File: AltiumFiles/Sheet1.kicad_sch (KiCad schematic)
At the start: 57 parts, among them J1 PJ-002A, U1 LM7805CT, U1A SS-104-G-2, U1RT SS-104-G-2, U2RT SS-104-G-2, Y1 ECS-100-18-1

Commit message: Kod za main
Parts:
- removed SW?: 2-1825910-7, FP-2-1825910-7-MFG, symbol Sheet1-altium-import:root_0_b8895f3f4cefb76e1819d2863dba89b
- added SW?: 2-1825910-7, FP-2-1825910-7-MFG, symbol Sheet1-altium-import:root_0_b8895f3f4cefb76e1819d2863dba89b
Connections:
- net GND: now also SW?.1, SW?.2, SW?.3, SW?.4

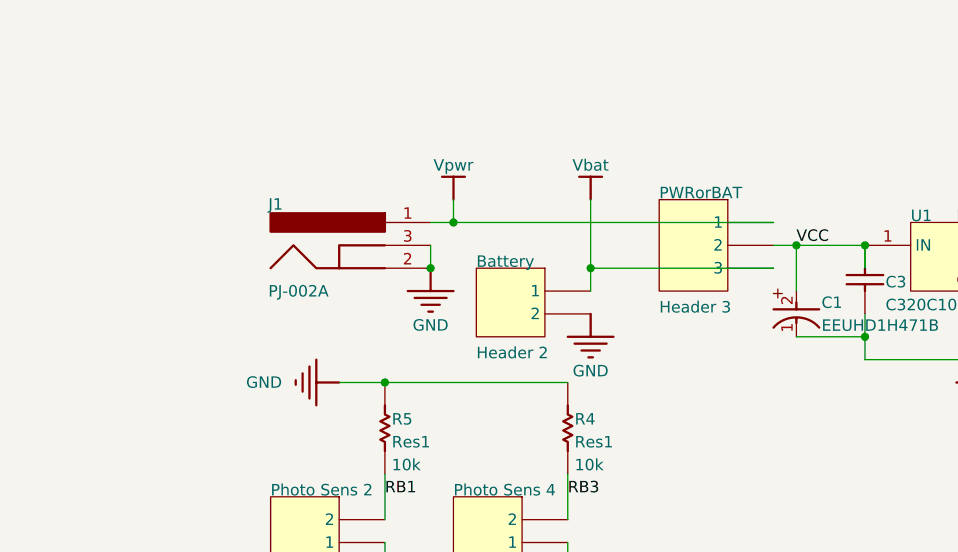
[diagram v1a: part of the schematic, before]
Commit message: End
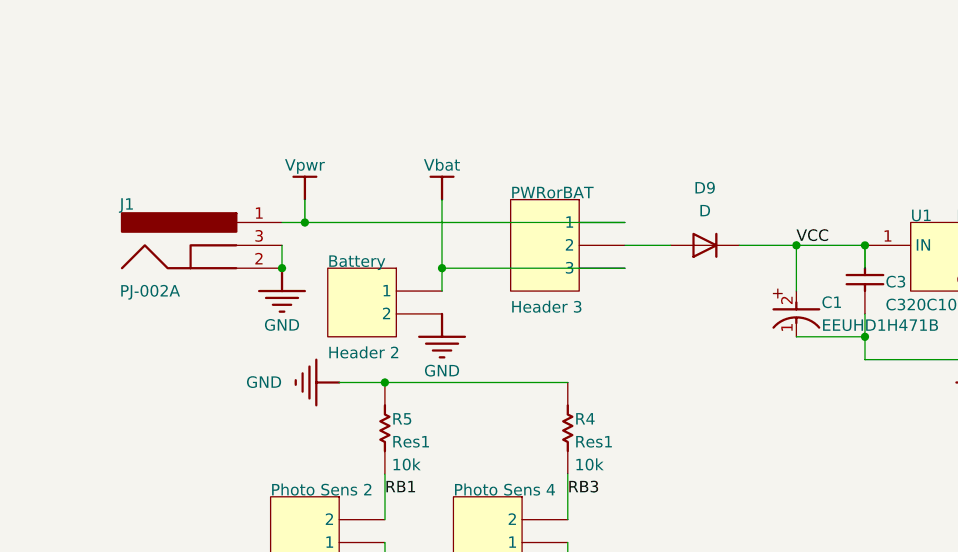
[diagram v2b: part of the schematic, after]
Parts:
- removed SW?: 2-1825910-7, FP-2-1825910-7-MFG, symbol Sheet1-altium-import:root_0_b8895f3f4cefb76e1819d2863dba89b
- added D9: D, symbol Device:D
- added SW?: 2-1825910-7, FP-2-1825910-7-MFG, symbol Sheet1-altium-import:root_0_b8895f3f4cefb76e1819d2863dba89b
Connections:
- net GND: now also SW?.1, SW?.2, SW?.3, SW?.4
- net VCC: now also D9.1 (K); no longer PWRorBAT.2
- new net: D9.2 (A), PWRorBAT.2
